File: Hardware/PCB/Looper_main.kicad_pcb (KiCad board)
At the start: 2 copper layers, 20 x 110.1 mm, 28 parts, among them J1 Out right, J11 Conn_01x06_Pin, J2 In left, J3 Trig Loop, J4 Out left, J5 In right, J6 Eurorack_Power, J8 Conn_01x05_Socket

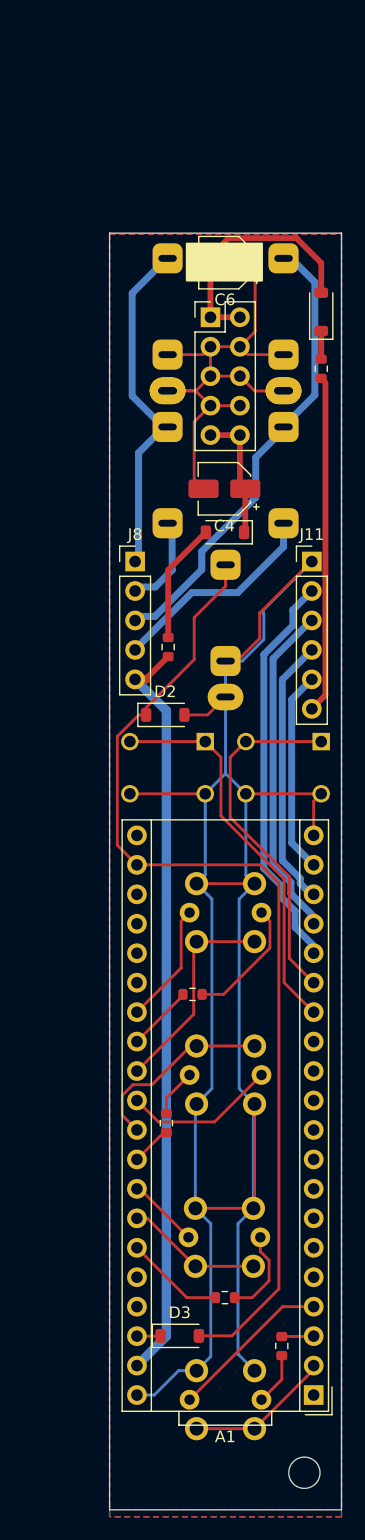
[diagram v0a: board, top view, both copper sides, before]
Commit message: Version 1.0 of hardware ordered
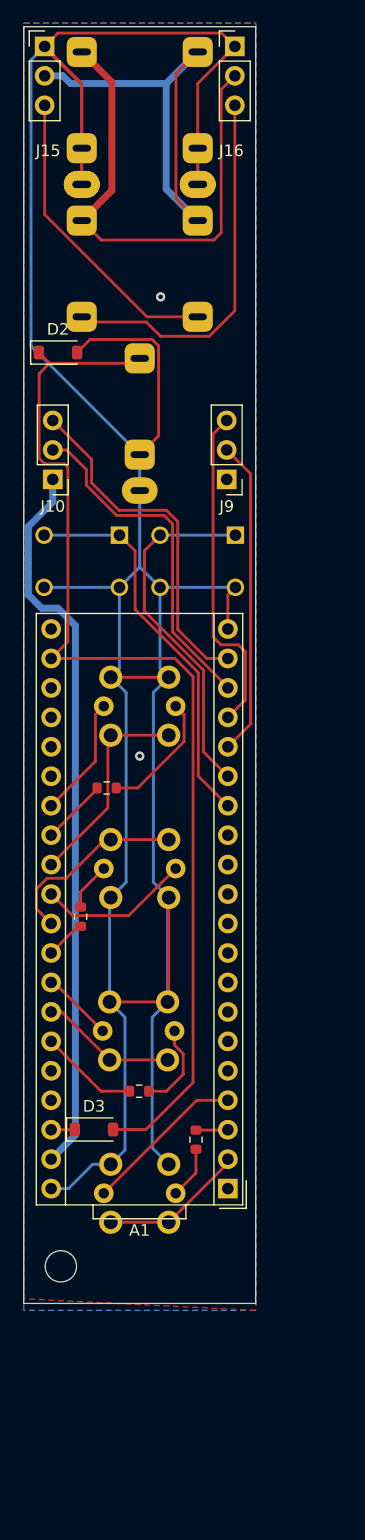
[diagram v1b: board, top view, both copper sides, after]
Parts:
- removed C4, C6: 10uF, Capacitor_SMD:CP_Elec_4x5.4
- removed D1, D4: 1N5819, Diode_SMD:D_SOD-123
- removed FB1, FB2: FerriteBead, Resistor_SMD:R_0603_1608Metric
- removed J11: Conn_01x06_Pin, Connector_PinHeader_2.54mm:PinHeader_1x06_P2.54mm_Vertical
- removed J6: Eurorack_Power, Connector_PinHeader_2.54mm:PinHeader_2x05_P2.54mm_Vertical
- removed J8: Conn_01x05_Socket, Connector_PinHeader_2.54mm:PinHeader_1x05_P2.54mm_Vertical
- added J10: Audio from Daisy, connect to J14, Connector_PinHeader_2.54mm:PinHeader_1x03_P2.54mm_Vertical, F.Cu at (-4.90, -98.5)
- added J15: Audio input, connect to J18, Connector_PinHeader_2.54mm:PinHeader_1x03_P2.54mm_Vertical, F.Cu at (-5.60, -135.8)
- added J16: Audio output, connect to J17, Connector_PinHeader_2.54mm:PinHeader_1x03_P2.54mm_Vertical, F.Cu at (10.8, -135.8)
- added J9: Audio to Daisy, connect to J13, Connector_PinHeader_2.54mm:PinHeader_1x03_P2.54mm_Vertical, F.Cu at (10.1, -98.5)
- moved D2 32.6 mm to (-4.45, -109.4)
- moved MOUNT1 27.5 mm to (-4.20, -30.6)
- moved J1 24.9 mm to (-2.40, -117.4)
- moved J4 24.9 mm to (-2.40, -130.4)
- moved J3 19.3 mm to (2.60, -104.0)
- moved S1 19.3 mm to (7.60, -91.4)
- moved S2 19.3 mm to (-2.40, -91.4)
- moved R1 19.3 mm to (2.55, -45.7)
- moved SW1 19.3 mm to (2.60, -78.9)
- moved SW2 19.3 mm to (2.60, -64.9)
- moved A1 19.3 mm to (10.2, -37.3)
- moved D3 19.3 mm to (-1.35, -42.4)
- moved R2 19.3 mm to (-2.50, -60.8)
- moved R3 19.3 mm to (-0.25, -71.8)
- moved R4 19.3 mm to (7.45, -41.5)
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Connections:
- J5 pad T: In Right -> (no net)
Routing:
- net GND: track 236.9 -> 278.1 mm, vias 0 -> 2
- net -12V: track 29.1 -> 0.00 mm
- net (no net): track 0.00 -> 26.3 mm
- net Net-(D1-A): track 21.9 -> 0.00 mm
- net In Left: track 29.6 -> 43.6 mm
- net Out Right: track 18.1 -> 31.9 mm
- net Out_R: track 17.5 -> 30.2 mm
- net Net-(D4-K): track 11.2 -> 0.00 mm
- net Net-(D4-A): track 10.4 -> 0.00 mm
- net In Right: track 7.79 -> 0.00 mm
- net Net-(A1-AUDIO_IN_L): track 34.5 -> 27.3 mm
- net Net-(A1-AUDIO_OUT_L): track 23.1 -> 29.8 mm
- net Net-(A1-ADC_INP10): track 87.3 -> 93.6 mm
- net Out Left: track 39.1 -> 43.7 mm
- net Net-(D1-K): track 2.42 -> 0.00 mm
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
